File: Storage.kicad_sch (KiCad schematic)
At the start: 12 parts, among them U5 KLM4G1FETE-B041

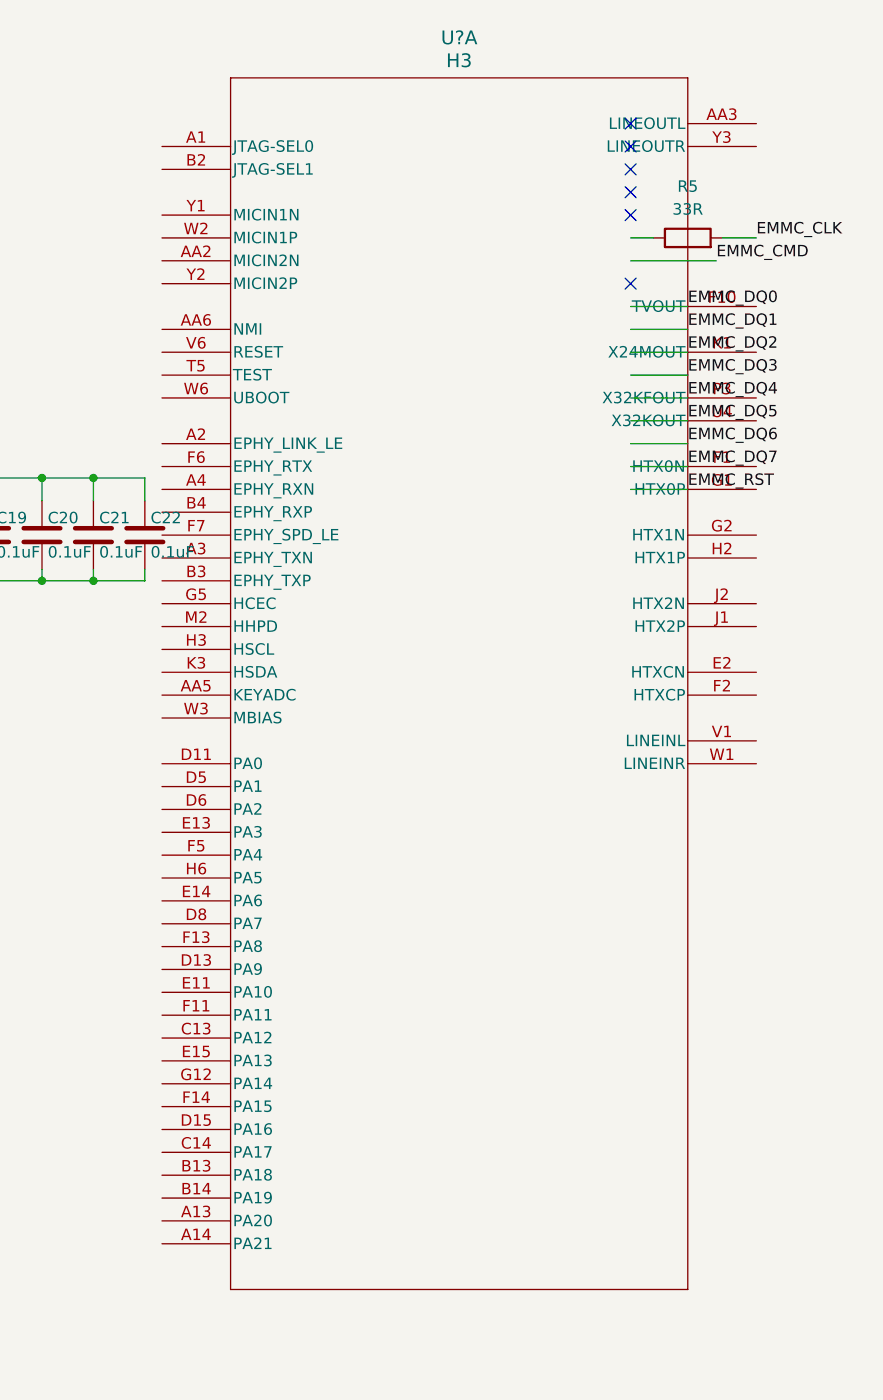
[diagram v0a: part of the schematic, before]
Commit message: changed some ethernet stuff
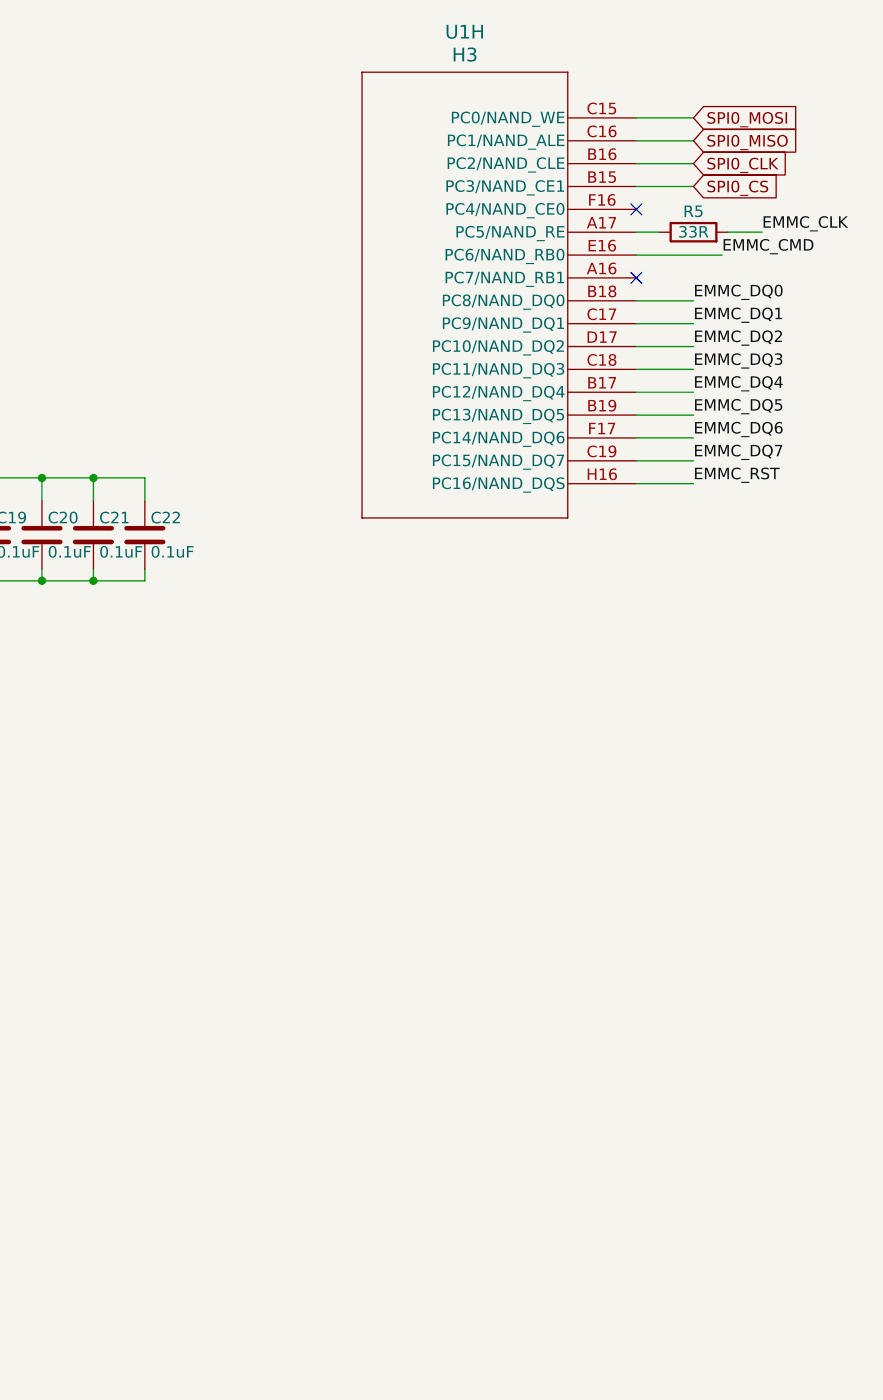
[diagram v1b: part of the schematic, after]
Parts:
- gave numbers to parts that had none: 1
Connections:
- net EMMC_CMD: now also U1.E16 (PC6/NAND_RB0)
- net EMMC_DQ0: now also U1.B18 (PC8/NAND_DQ0)
- net EMMC_DQ1: now also U1.C17 (PC9/NAND_DQ1)
- net EMMC_DQ2: now also U1.D17 (PC10/NAND_DQ2)
- net EMMC_DQ3: now also U1.C18 (PC11/NAND_DQ3)
- net EMMC_DQ4: now also U1.B17 (PC12/NAND_DQ4)
- net EMMC_DQ5: now also U1.B19 (PC13/NAND_DQ5)
- net EMMC_DQ6: now also U1.F17 (PC14/NAND_DQ6)
- net EMMC_DQ7: now also U1.C19 (PC15/NAND_DQ7)
- net EMMC_RST: now also U1.H16 (PC16/NAND_DQS)
- net at R5.1: now also U1.A17 (PC5/NAND_RE)
- new net SPI0_CLK: U1.B16 (PC2/NAND_CLE)
- new net SPI0_CS: U1.B15 (PC3/NAND_CE1)
- new net SPI0_MISO: U1.C16 (PC1/NAND_ALE)
- new net SPI0_MOSI: U1.C15 (PC0/NAND_WE)
- no-connect marks 127 -> 123
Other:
- moved on the sheet: R5
